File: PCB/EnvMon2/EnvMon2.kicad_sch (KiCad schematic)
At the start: 37 parts, among them J1 USB-C, J2 DC, J3 TEMP, J4 Shelly, M1 OLED1.5-RGB, SW1 SW_Push, SW2 SW_Push, SW3 SW_Push, U1 LMR16006+FB, U2 SCD41, U3 FT231XQ, U4 ESP32-PICO-MINI-02, U5 QR, U6 VEML3235SL-RA

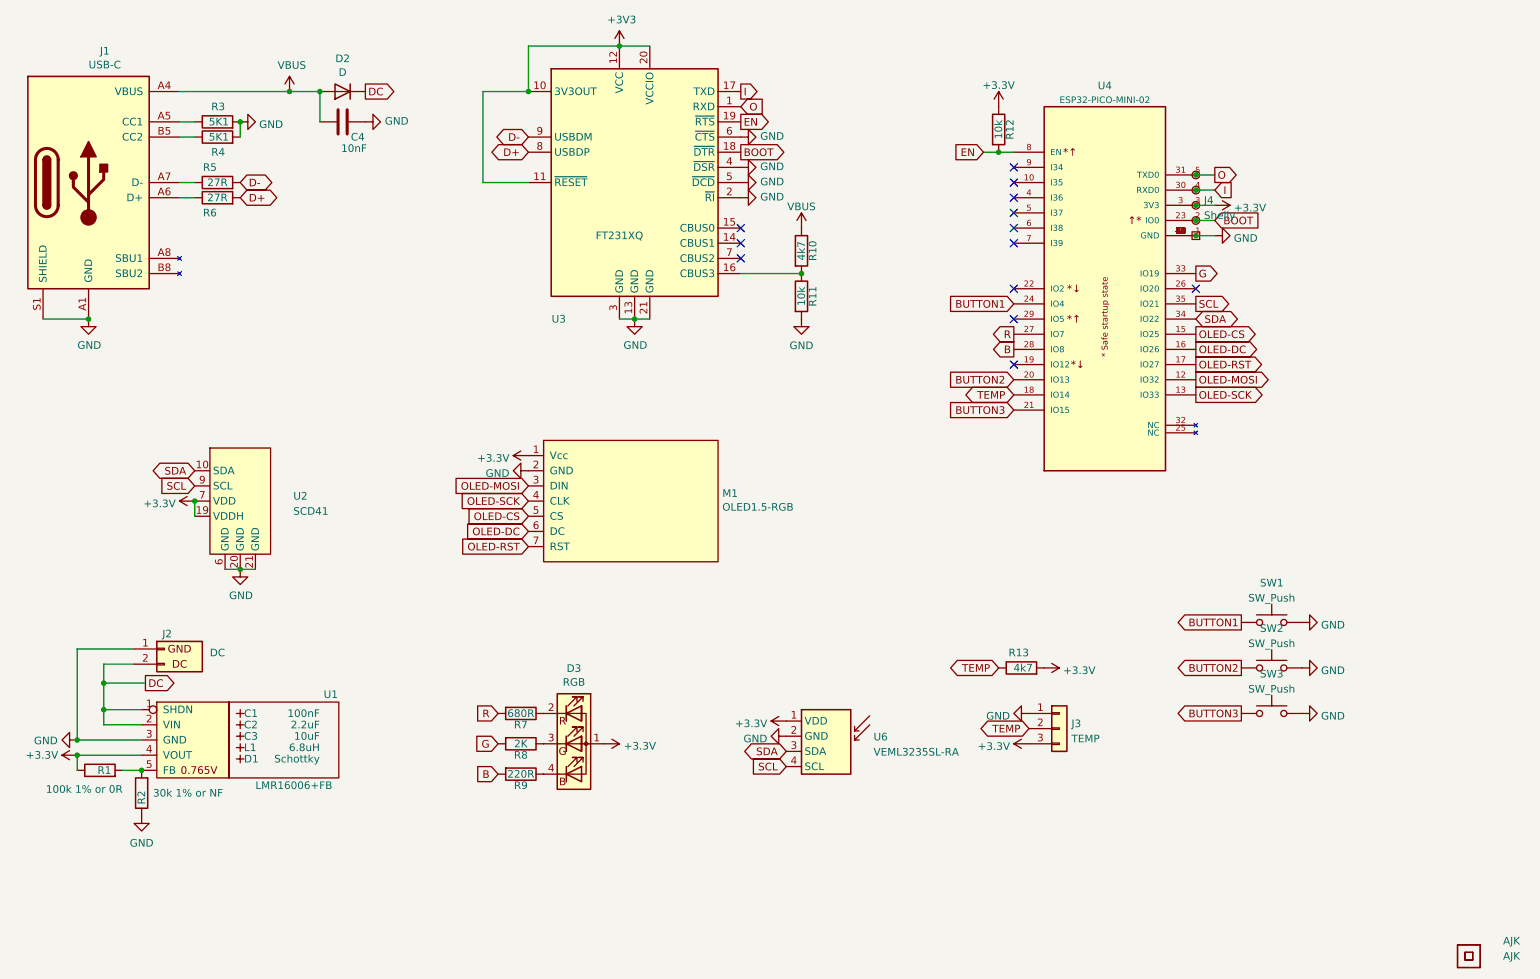
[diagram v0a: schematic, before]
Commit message: Library update
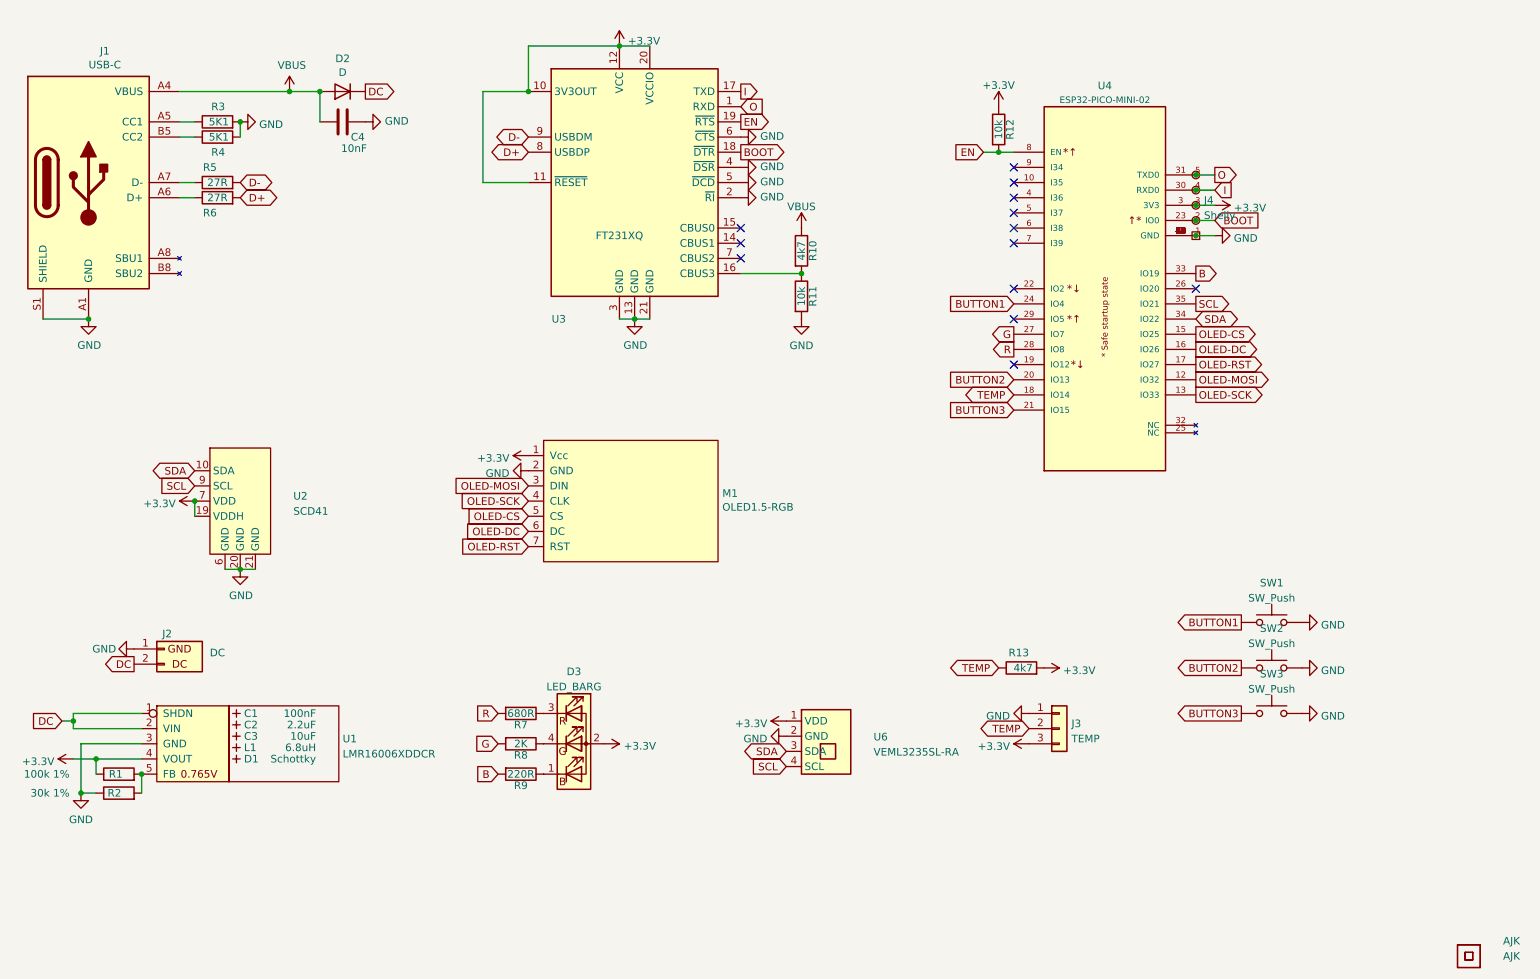
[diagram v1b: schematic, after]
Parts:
- removed D3: RGB, RevK:LED-RGB-1.6x1.6, symbol Device:LED_ARGB
- added D3: LED_BARG, RevK:MHS190RGBCT, symbol Device:LED_BARG
- C1: footprint RevK:C_0603_ -> RevK:Hidden; LCSC Part # (none) -> C30926
- C2: footprint RevK:C_0805_ -> RevK:Hidden; LCSC Part # (none) -> C19110
- C3: footprint RevK:C_0805_ -> RevK:Hidden; LCSC Part # (none) -> C17024
- D1: footprint RevK:D_1206_ -> RevK:Hidden; JLCPCB Rotation Offset (none) -> 180; LCSC Part # (none) -> C143805; Part No CD1206-B2100 -> (none)
- J1: LCSC Part # (none) -> C709357
- L1: footprint RevK:L_4x4_ -> RevK:Hidden; LCSC Part # (none) -> C354575; Manufacturer Laird -> (none); Part No TYA4020 -> (none)
- R1: value 100k 1% or 0R -> 100k 1%; LCSC Part # (none) -> C14675
- R2: value 30k 1% or NF -> 30k 1%; LCSC Part # (none) -> C100001
- U1: value LMR16006+FB -> LMR16006XDDCR; footprint RevK:RegulatorBlockFB -> RevK:SOT-23-Thin-6-Reg; LCSC Part # (none) -> C87080
- U3: footprint RevK:QFN-20-1EP_4x4mm_P0.5mm_EP2.5x2.5mm -> RevK:JLC-QFN-20-1EP_4x4mm_P0.5mm_EP2.5x2.5m
- U4: LCSC Part # (none) -> C2980306; Part No (none) -> ESP32-PICO-MINI-02-N8R2
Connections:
- net B: now also U4.33 (IO19); no longer U4.28 (IO8)
- net G: now also U4.27 (IO7); no longer U4.33 (IO19)
- net R: now also U4.28 (IO8); no longer U4.27 (IO7)
- net at R9.1: now also D3.1 (BK)
- net at R7.1: now also D3.3 (RK)
- net at R8.1: now also D3.4 (GK)
- net +3V3 renamed +3.3V
- net +3.3V: now also D3.2 (A)
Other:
- moved on the sheet: J4

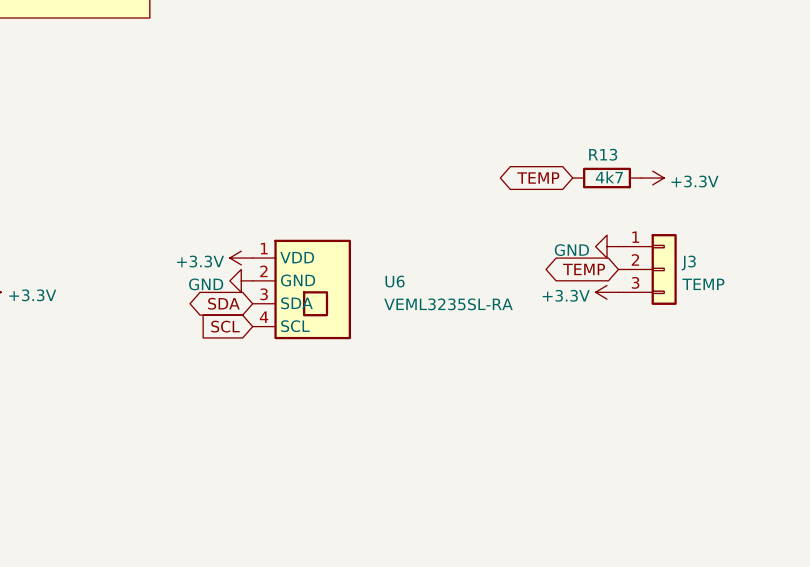
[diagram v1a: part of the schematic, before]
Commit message: Revised production files
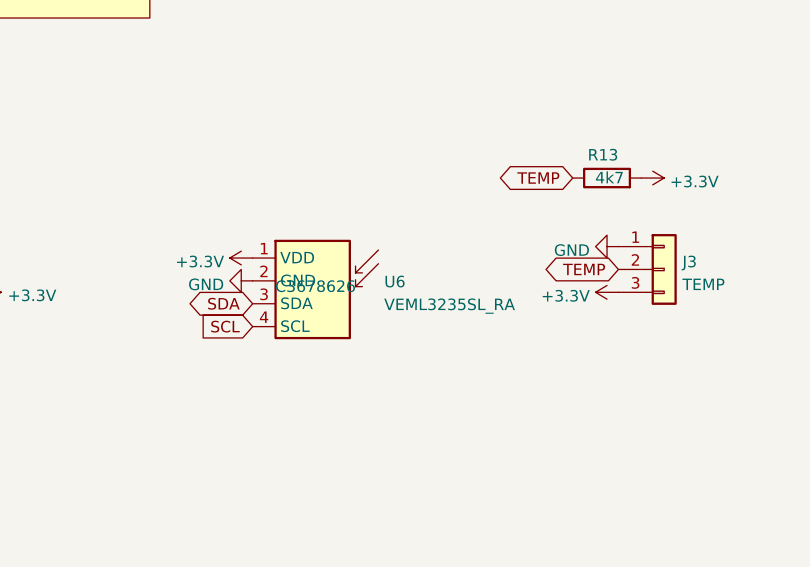
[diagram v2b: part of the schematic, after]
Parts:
- removed U6: VEML3235SL-RA, RevK:VEML3235SL-RA, symbol RevK:VEML3235SL
- added U6: VEML3235SL_RA, RevK:VEML3235SL-RA, symbol RevK:VEML3235SL_RA
- C1: footprint RevK:Hidden -> RevK:C_0603_
- C2, C3: footprint RevK:Hidden -> RevK:C_0805_
- D1: footprint RevK:Hidden -> RevK:D_1206_; JLCPCB Rotation Offset 180 -> (none)
- D2: LCSC Part # (none) -> C143805
- L1: footprint RevK:Hidden -> RevK:L_4x4_
- U1: Manufacturer TI -> (none); Part No LMR16006YQ3 -> (none)
- U3: footprint RevK:JLC-QFN-20-1EP_4x4mm_P0.5mm_EP2.5x2.5m -> RevK:QFN-20-1EP_4x4mm_P0.5mm_EP2.5x2.5mm; JLCPCB Rotation Offset (none) -> -90
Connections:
- net +3.3V: now also U6.1 (VDD)
- net GND: now also U6.2 (GND)
- net SCL: now also U6.4 (SCL)
- net SDA: now also U6.3 (SDA)
